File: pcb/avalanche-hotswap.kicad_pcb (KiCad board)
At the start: 2 copper layers, 173 x 137.5 mm, 140 parts, among them J1 TRRS, J3 OLED, P1 i2c_pin, P2 i2c_pin, SW0 SW_Push, SW1 SW_Push, SW10 SW_Push, SW11 SW_Push, SW12 SW_Push, SW13 SW_Push, SW14 SW_Push, SW15 SW_Push, SW16 SW_Push, SW17 SW_Push, SW18 SW_Push, SW2 SW_Push, SW20 SW_Push, SW21 SW_Push, SW22 SW_Push, SW23 SW_Push, SW24 SW_Push, SW25 SW_Push, SW26 SW_Push, SW27 SW_Push, SW28 SW_Push, SW29 SW_Push, SW3 SW_Push, SW30 SW_Push, SW31 SW_Push, SW32 SW_Push, SW4 SW_Push, SW5 SW_Push, SW6 SW_Push, SW7 SW_Push, SW8 SW_Push, SW9 SW_Push, U1 ProMicro

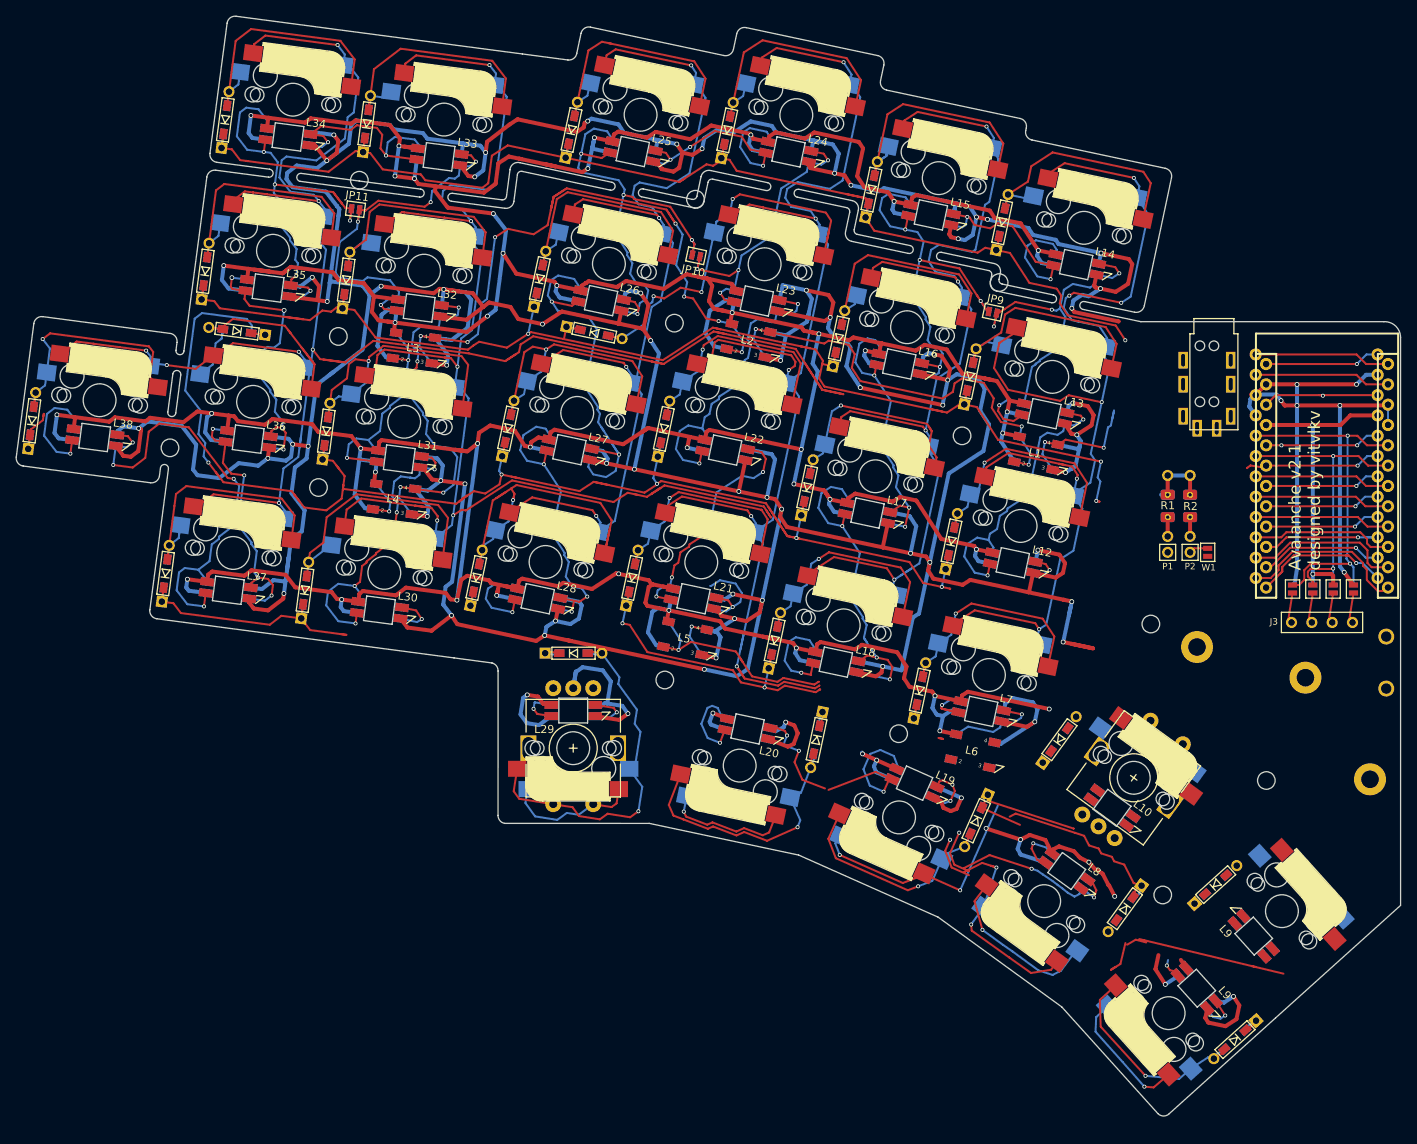
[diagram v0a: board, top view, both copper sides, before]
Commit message: Work in progress
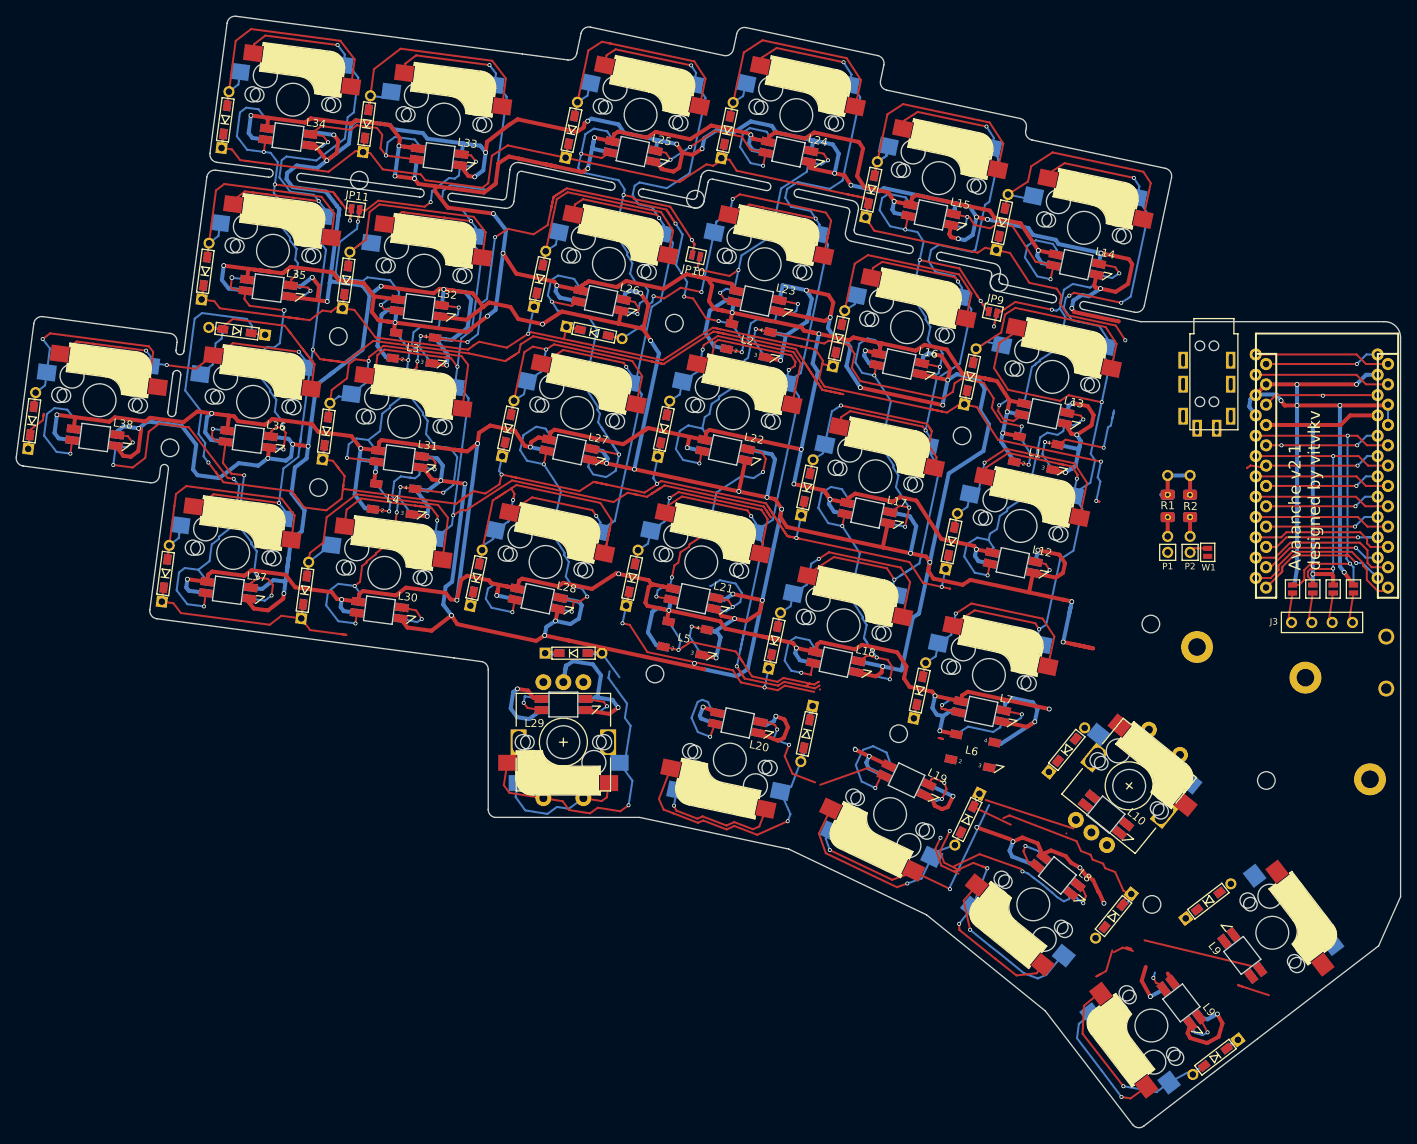
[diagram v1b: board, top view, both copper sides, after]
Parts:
- moved D32 3.28 mm to (199.9, 152.7), turned to 217.5 degrees
- moved SW32 2.96 mm to (207.0, 137.1), turned to 127.5 degrees
- moved L9 2.81 mm to (203.2, 140.0), turned to 127.5 degrees
- moved L9 2.66 mm to (195.6, 145.9), turned to 307.5 degrees
- moved SW32 2.66 mm to (191.9, 148.7), turned to 307.5 degrees
- moved D32 2.25 mm to (199.0, 133.2), turned to 37.5 degrees
- moved HM1 1.79 mm to (192.0, 133.6), turned to 340.5 degrees
- moved D31 1.70 mm to (187.1, 135.0), turned to 231 degrees
- moved D26 1.58 mm to (181.3, 114.3), turned to 51 degrees
- moved SW29 1.44 mm to (139.2, 115.5)
- moved ENC3 1.44 mm to (118.4, 113.3)
- moved L29 1.44 mm to (118.4, 108.6)
- moved SW28 1.44 mm to (118.4, 113.3)
- moved D29 1.44 mm to (148.8, 112.3)
- moved HM13 1.44 mm to (129.8, 104.8)
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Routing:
- net row4: track 82.3 -> 70.7 mm
- net encA: track 21.4 -> 33.0 mm
- net Net-(L5-Pad2): track 27.8 -> 28.6 mm
- net row3: track 97.8 -> 97.0 mm, vias 2 -> 3
- net GND: vias 71 -> 70
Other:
- board size 173 x 137.5 mm -> 173 x 138.9 mm
